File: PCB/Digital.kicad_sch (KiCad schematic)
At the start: 15 parts, among them IC1 MAX3051ESA+, J2 ICSP, J3 DE9_Plug_MountingHoles, J4 Conn_Coaxial, U1 PIC18F2580T-I/SO, Y2 ABLS-8.000MHZ-B2-T

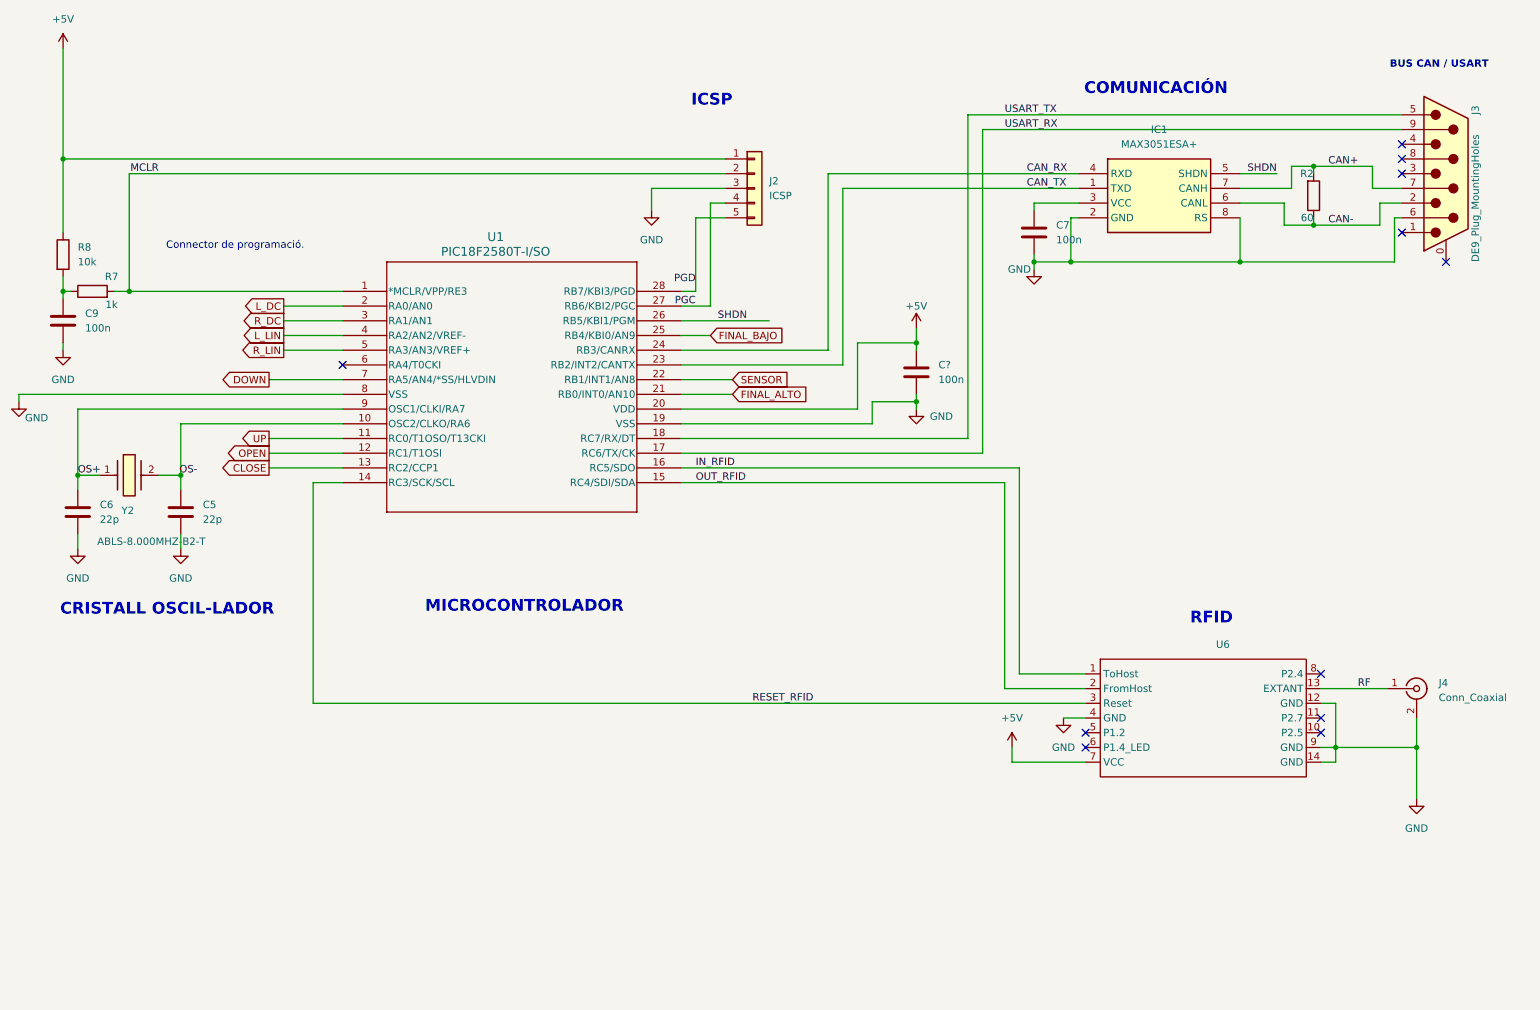
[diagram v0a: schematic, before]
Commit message: Add files via upload
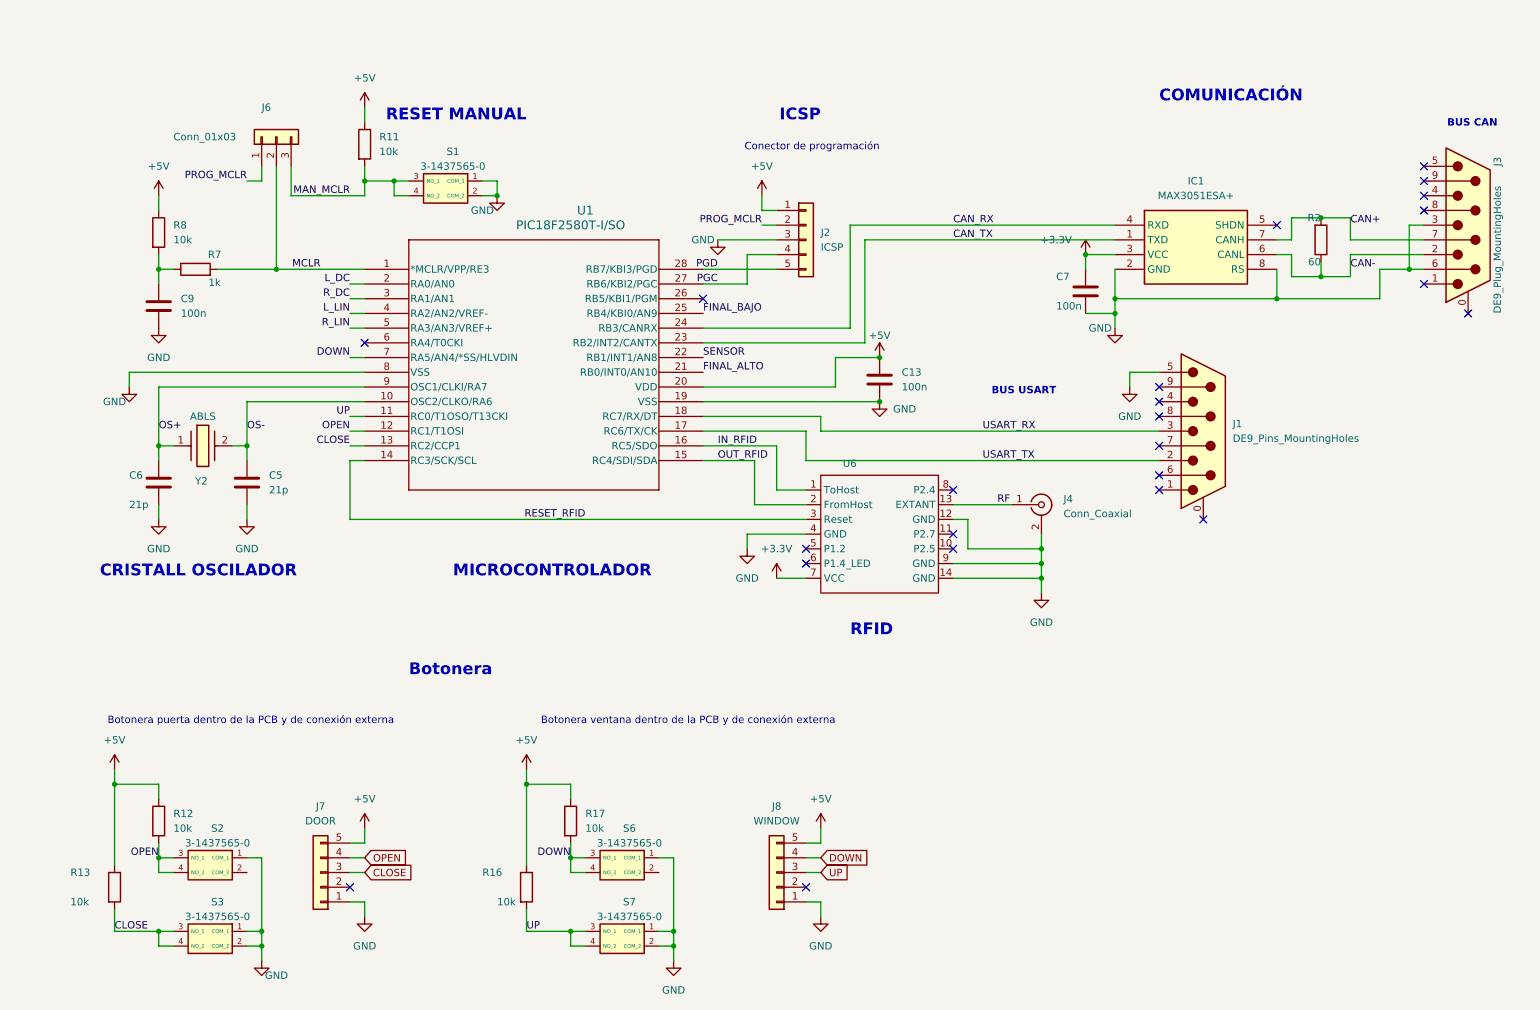
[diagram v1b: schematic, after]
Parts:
- removed C?: 100n, symbol Device:C
- added C13: 100n, Capacitor_SMD:C_1206_3216Metric, symbol Device:C
- added J1: DE9_Pins_MountingHoles, Connector_Dsub:DSUB-9_Pins_Horizontal_P2.77x2.84mm_EdgePinOffset4.94mm_Housed_MountingHolesOffset4.94mm, symbol Connector:DE9_Pins_MountingHoles
- added J6: Conn_01x03, Connector_PinHeader_2.54mm:PinHeader_1x03_P2.54mm_Vertical, symbol Connector_Generic:Conn_01x03
- added J7: DOOR, Connector_PinHeader_2.54mm:PinHeader_1x05_P2.54mm_Vertical, symbol Connector_Generic:Conn_01x05
- added J8: WINDOW, Connector_PinHeader_2.54mm:PinHeader_1x05_P2.54mm_Vertical, symbol Connector_Generic:Conn_01x05
- added R11, R12, R13, R16, R17: 10k, Capacitor_SMD:C_1206_3216Metric, symbol Device:R
- added S1, S2, S3, S6, S7: 3-1437565-0, 3-1437565-0:314375650, symbol 3-1437565-0:3-1437565-0
- C5, C6: value 22p -> 21p; footprint (none) -> Capacitor_SMD:C_0201_0603Metric
- C7, C9: footprint (none) -> Capacitor_SMD:C_1206_3216Metric
- IC1: footprint SOIC127P600X175-8N -> MAX3051ESA+:SOIC127P600X175-8N
- J2: footprint (none) -> Connector_PinHeader_2.54mm:PinHeader_1x05_P2.54mm_Vertical
- J3: footprint Connector_Dsub:DSUB-9_Female_Horizontal_P2.77x2.84mm_EdgePinOffset4.94mm_Housed_MountingHolesOffset7.48mm -> Connector_Dsub:DSUB-9_Pins_Horizontal_P2.77x2.84mm_EdgePinOffset4.94mm_Housed_MountingHolesOffset4.94mm
- J4: footprint (none) -> Connector_Coaxial:BNC_TEConnectivity_1478035_Horizontal
- R7: footprint (none) -> Resistor_SMD:R_0603_1608Metric
- R8: footprint (none) -> Resistor_SMD:R_1206_3216Metric
- U1: footprint SOIC28-W_MC_MCH -> PIC18F2580T_I_SO:SOIC28-W_MC_MCH
- Y2: value ABLS-8.000MHZ-B2-T -> ABLS; footprint ABLS8000MHZB2T -> ABLS8000MHZB2T:ABLS8000MHZB2T
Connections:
- net +5V: now also C13.1, J7.5 (Pin_5), J8.5 (Pin_5), R11.1, R12.1, R13.1, R16.1, R17.1; no longer U6.7 (VCC)
- net CLOSE: now also J7.3 (Pin_3), R13.2, S3.3 (NO_1), S3.4 (NO_2)
- net DOWN: now also J8.4 (Pin_4), R17.2, S6.3 (NO_1), S6.4 (NO_2)
- net GND: now also J3.3, C13.2, J1.5, J7.1 (Pin_1), J8.1 (Pin_1), S1.1 (COM_1), S1.2 (COM_2), S2.1 (COM_1), S3.1 (COM_1), S3.2 (COM_2), S6.1 (COM_1), S7.1 (COM_1), S7.2 (COM_2)
- net MCLR: now also J6.2 (Pin_2); no longer J2.2 (Pin_2)
- net OPEN: now also J7.4 (Pin_4), R12.2, S2.3 (NO_1), S2.4 (NO_2)
- net UP: now also J8.3 (Pin_3), R16.2, S7.3 (NO_1), S7.4 (NO_2)
- net USART_RX: now also U1.18 (RC7/RX/DT), J1.3; no longer J3.9, U1.17 (RC6/TX/CK)
- net USART_TX: now also U1.17 (RC6/TX/CK), J1.2; no longer J3.5, U1.18 (RC7/RX/DT)
- net +3.3V: now reaches C7.1, IC1.3 (VCC)
- net +3.3V: now also U6.7 (VCC)
- net SHDN: no longer names the net of IC1.5 (SHDN)
- net SHDN: no longer U1.26 (RB5/KBI1/PGM)
- new net MAN_MCLR: J6.3 (Pin_3), R11.2, S1.3 (NO_1), S1.4 (NO_2)
- new net PROG_MCLR: J2.2 (Pin_2), J6.1 (Pin_1)
- no-connect marks 11 -> 23
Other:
- note added: "BUS CAN"
- note added: "BUS USART"
- note added: "Botonera"
- note added: "Botonera puerta dentro de la PCB y de conexión externa"
- note added: "Botonera ventana dentro de la PCB y de conexión externa"
- note added: "CRISTALL OSCILADOR"
- note added: "Conector de programación"
- note added: "RESET MANUAL"
- note removed: "BUS CAN / USART"
- note removed: "CRISTALL OSCIL-LADOR"
- note removed: "Connector de programació."
- moved on the sheet: C5, C6, C7, C9, IC1, J2, J3, J4, R2, R7, R8, U1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
